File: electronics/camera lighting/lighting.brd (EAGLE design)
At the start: 26 x 26 mm, 10 parts

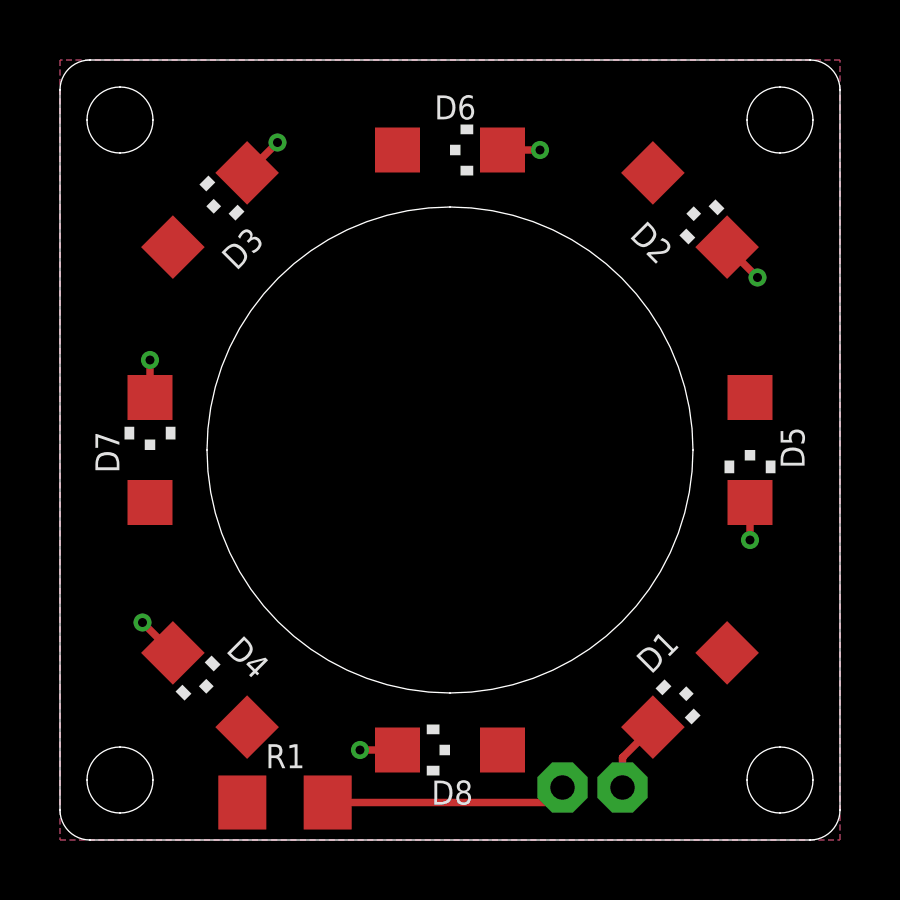
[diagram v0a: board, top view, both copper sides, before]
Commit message: pre-production PCBs
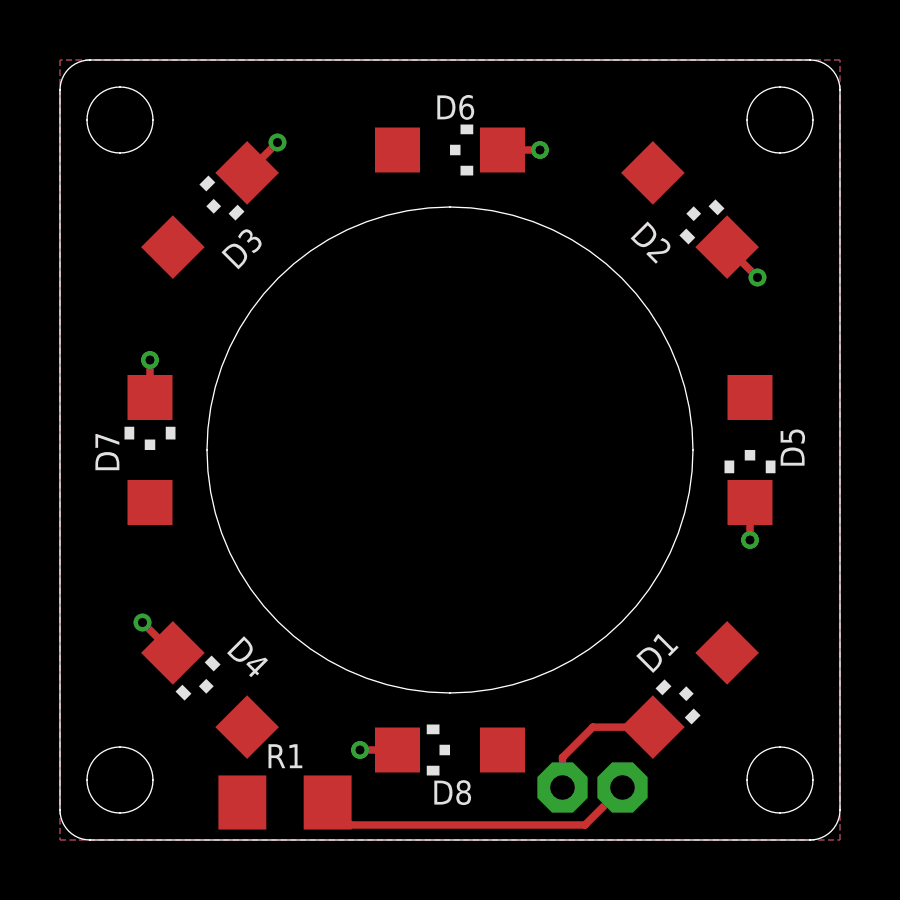
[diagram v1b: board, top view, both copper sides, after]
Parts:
- renumbered P1 to PWR
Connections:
- net 5V: now also PWR.2; no longer PWR.1
- net GND: now also PWR.1; no longer PWR.2
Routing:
- net 5V: track 8.04 -> 10.7 mm
- net GND: track 11.7 -> 13.7 mm
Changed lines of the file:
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@@
 <attribute name="VALUE" x="14.27" y="5.54" size="1.27" layer="27" rot="R180"/>
 </element>
-<element name="P1" library="jst-ph" package="JST-PH2" value="" x="17.75" y="1.75" smashed="yes" rot="MR0"/>
+<element name="PWR" library="jst-ph" package="JST-PH2" value="" x="17.75" y="1.75" smashed="yes" rot="MR0"/>
 </elements>
 <signals>
 <signal name="5V">
 <contactref element="R1" pad="2"/>
-<contactref element="P1" pad="1"/>
-<wire x1="8.922" y1="1.25" x2="16.25" y2="1.25" width="0.25" layer="1"/>
-<wire x1="16.25" y1="1.25" x2="16.75" y2="1.75" width="0.25" layer="1"/>
+<contactref element="PWR" pad="2"/>
+<wire x1="18.75" y1="1.75" x2="17.5" y2="0.5" width="0.25" layer="1"/>
+<wire x1="17.5" y1="0.5" x2="9.672" y2="0.5" width="0.25" layer="1"/>
+<wire x1="9.672" y1="0.5" x2="8.922" y2="1.25" width="0.25" layer="1"/>
 </signal>
 <signal name="GND">
@@
 <vertex x="0" y="26"/>
 </polygon>
-<contactref element="P1" pad="2"/>
 <via x="2.75" y="7.25" extent="1-16" drill="0.3"/>
 <via x="3" y="16" extent="1-16" drill="0.3"/>
@@
 <wire x1="23.249996875" y1="18.75" x2="23.25" y2="18.75" width="0.25" layer="1"/>
 <wire x1="23" y1="11.25" x2="23" y2="10" width="0.25" layer="1"/>
-<wire x1="19.7625625" y1="3.7625625" x2="18.75" y2="2.75" width="0.25" layer="1"/>
-<wire x1="18.75" y1="2.75" x2="18.75" y2="1.75" width="0.25" layer="1"/>
 <via x="10" y="3" extent="1-16" drill="0.3"/>
 <wire x1="11.25" y1="3" x2="10" y2="3" width="0.25" layer="1"/>
+<contactref element="PWR" pad="1"/>
+<wire x1="19.7625625" y1="3.7625625" x2="17.7625625" y2="3.7625625" width="0.25" layer="1"/>
+<wire x1="17.7625625" y1="3.7625625" x2="16.75" y2="2.75" width="0.25" layer="1"/>
+<wire x1="16.75" y1="2.75" x2="16.75" y2="1.75" width="0.25" layer="1"/>
 </signal>
 <signal name="COMMON">
